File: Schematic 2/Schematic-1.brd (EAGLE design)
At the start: 127.2 x 80.2 mm, 37 parts, among them IC1 7805T, IC3 MCP23017SO, Q1 BSS138, Q2 BSS138, U2 LMV358, U3 LMV324

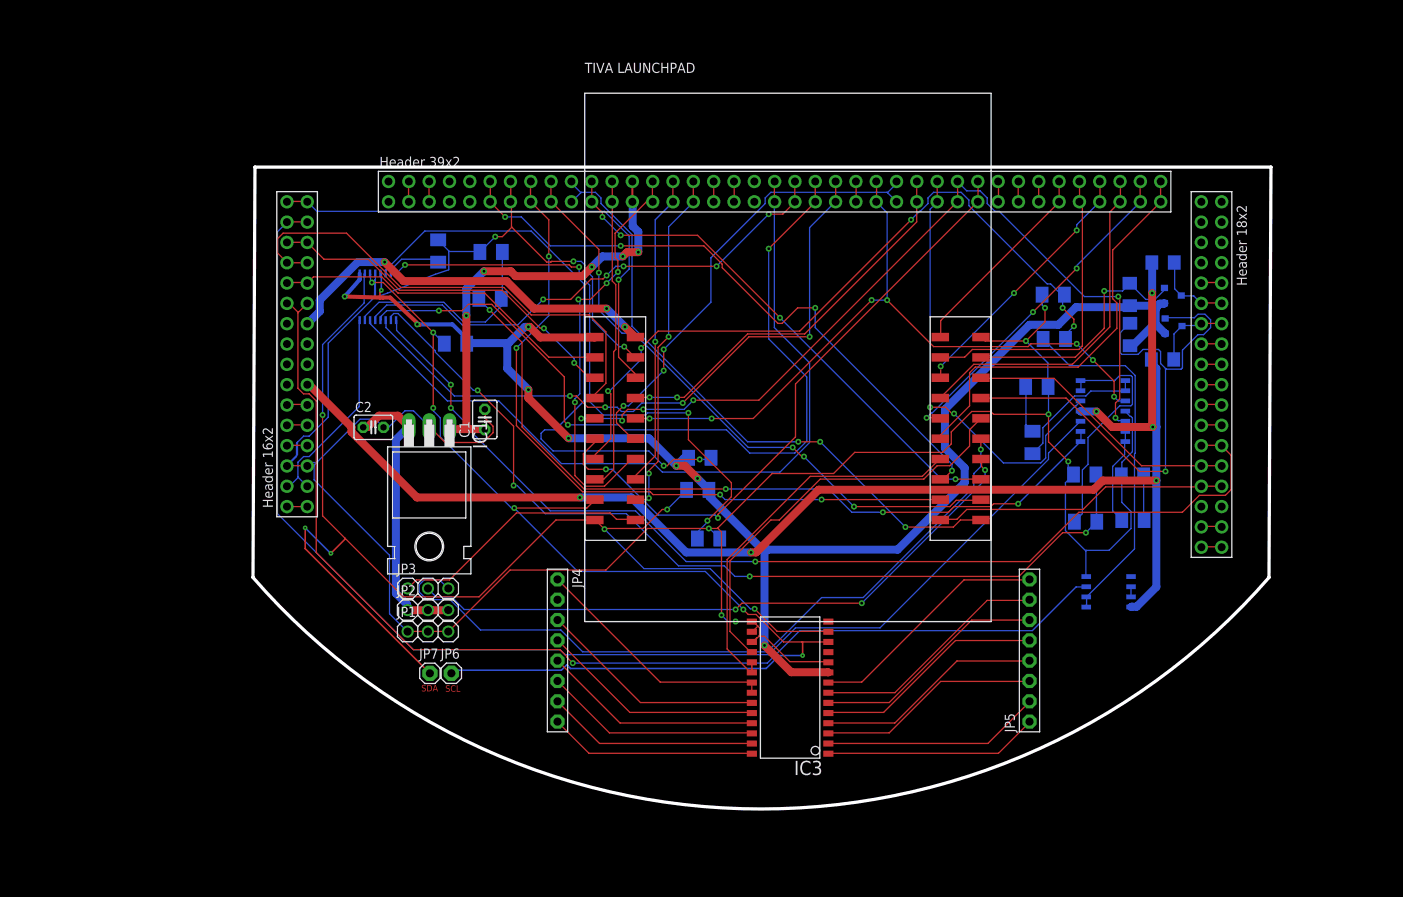
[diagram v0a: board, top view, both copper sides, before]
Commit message: Final tweaks to plugable Tiva board
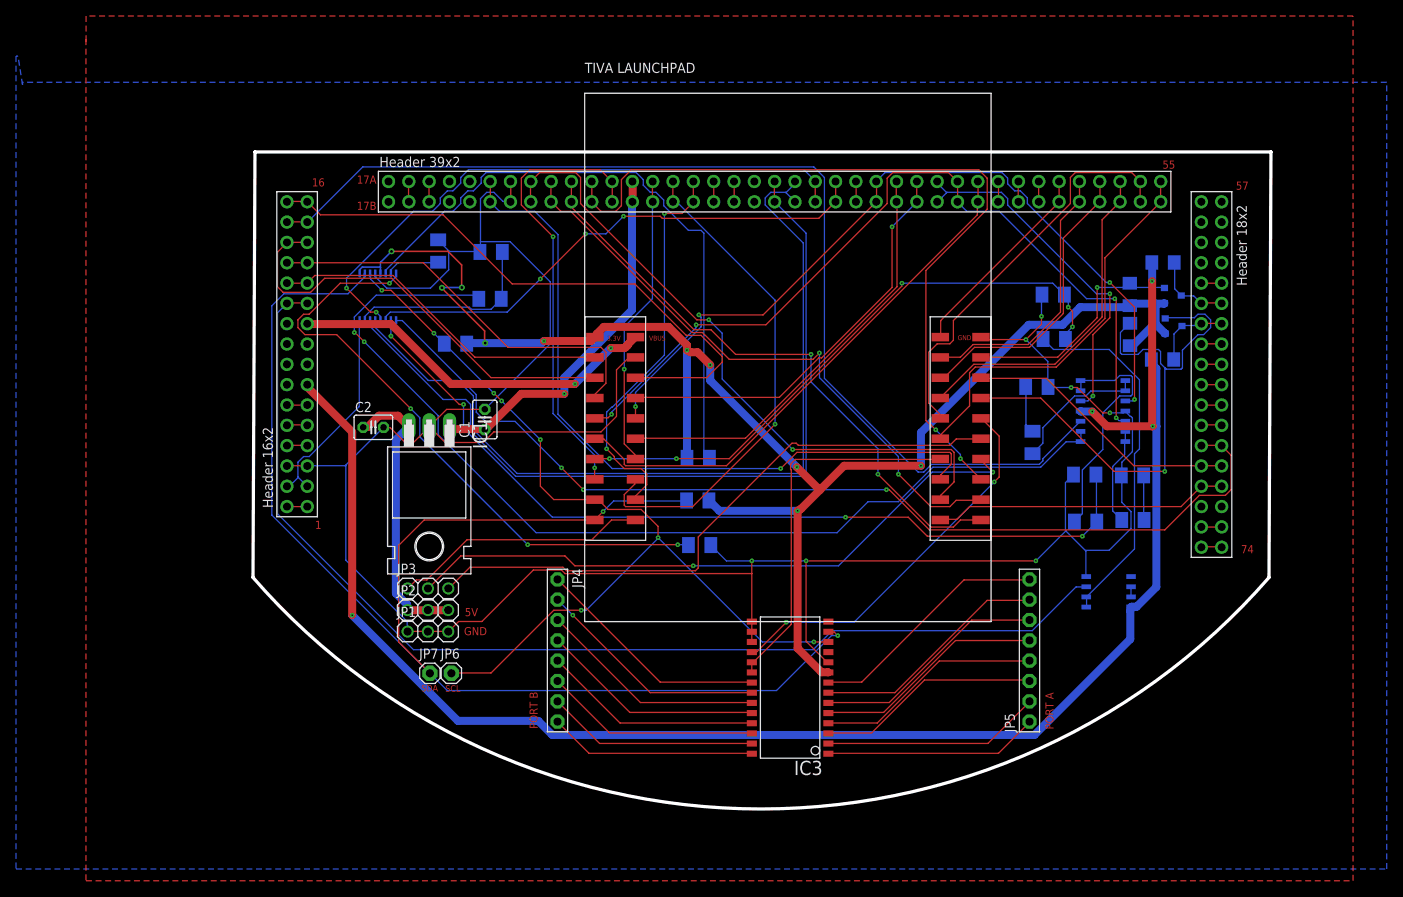
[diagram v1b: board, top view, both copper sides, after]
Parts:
- moved R4 1.38 mm to (55.8, 4.18)
- moved R1 1.32 mm to (55.5, 9.76)
- moved R3 0.20 mm to (55.6, 15.1)
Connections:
- new net N$9: IC3.22, JP4.2
- net N$3: no longer IC3.22
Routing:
- net 37: track 63.5 -> 107.0 mm, vias 5 -> 0
- net 27: track 65.9 -> 100.7 mm, vias 4 -> 2
- net N2: track 97.4 -> 127.4 mm, vias 4 -> 2
- net SCL: track 143.5 -> 113.9 mm, vias 6 -> 8
- net N$9: track 0.00 -> 29.1 mm, vias 0 -> 1
- net 38: track 102.8 -> 75.6 mm, vias 3 -> 2
- net SDA: track 153.8 -> 179.7 mm, vias 6 -> 2
- net 5V1: track 182.7 -> 207.3 mm, vias 6 -> 4
- net 15: track 159.7 -> 135.4 mm
- net 31: track 39.2 -> 62.9 mm
- net 39: track 82.9 -> 65.4 mm, vias 4 -> 3
- net 28: track 39.2 -> 56.4 mm, vias 0 -> 2
- net PB4: track 90.6 -> 74.9 mm
- net PB7: track 92.6 -> 77.2 mm, vias 1 -> 0
- net 30: track 52.1 -> 36.8 mm, vias 4 -> 1
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- added copper zone on layer 1, net GND
- added copper zone on layer 16, net GND
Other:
- board size 127.2 x 80.2 mm -> 127.2 x 82.1 mm
- board text added: "1"
- board text added: "16"
- board text added: "17A"
- board text added: "17B"
- board text added: "3.3V"
- board text added: "55"
- board text added: "57"
- board text added: "5V"
- board text added: "74"
- board text added: "GND"
- board text added: "PORT A"
- board text added: "PORT B"
- board text added: "VBUS"
